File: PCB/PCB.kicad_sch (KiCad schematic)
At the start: 45 parts, among them J1 6V, J10 GND, J11 GND, J12 VBUS, J13 GND, J14 3V3, J15 6V, J16 GND, J2 GND, J3 12V, J4 GND, J5 vREF, J6 GND, J7 6V, J8 5V, J9 GND, U1 TPS565208, U2 OPA192ID, U3 ADP7142AUJZ-5.0, U4 MCP1826S-3302E/DB

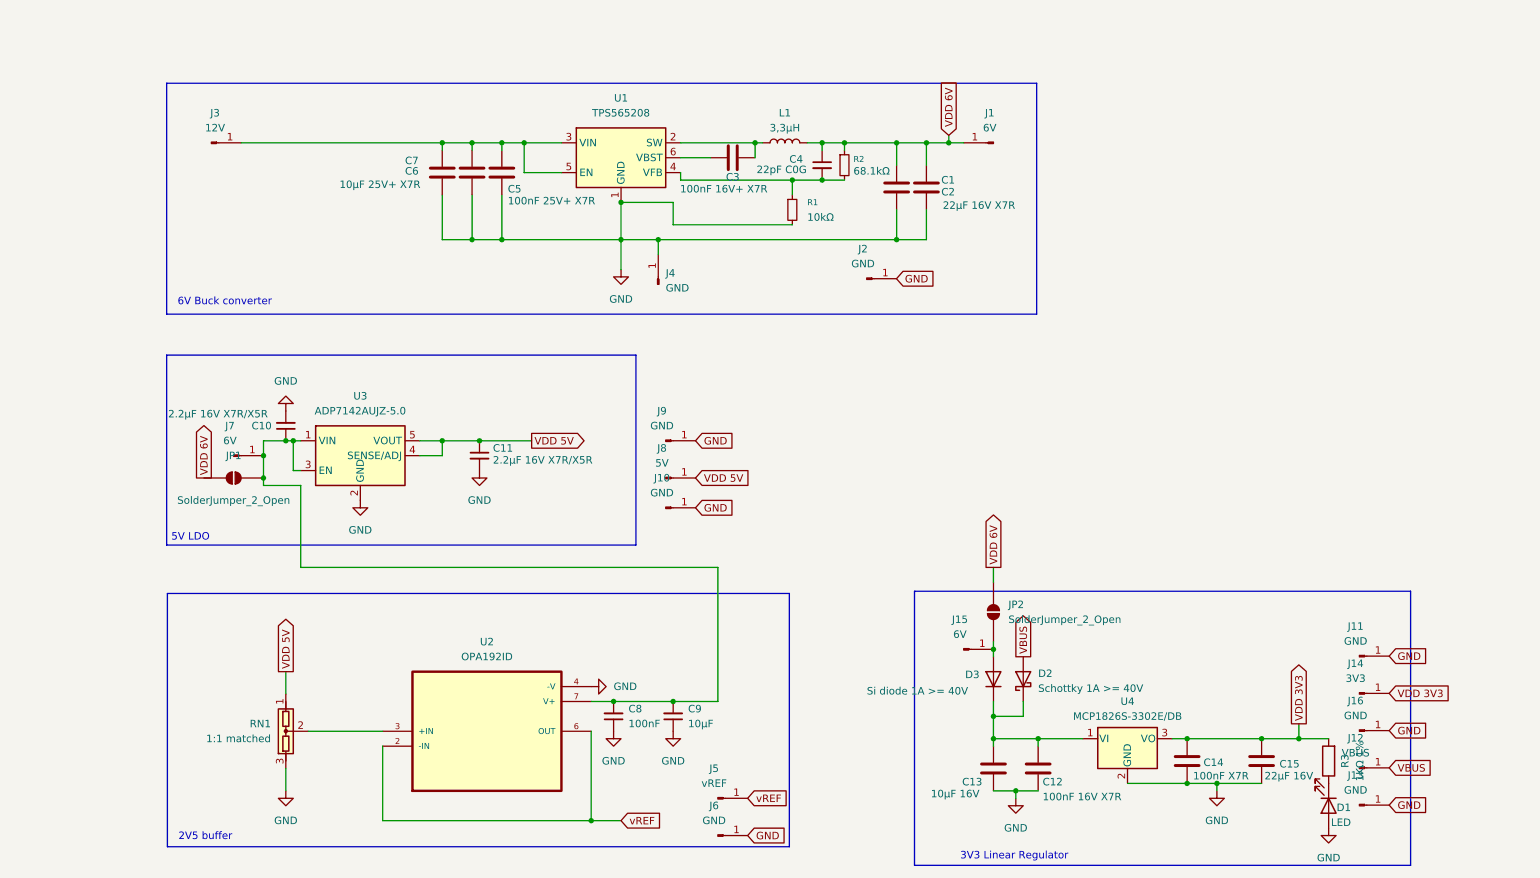
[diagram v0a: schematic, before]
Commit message: schematic rethought
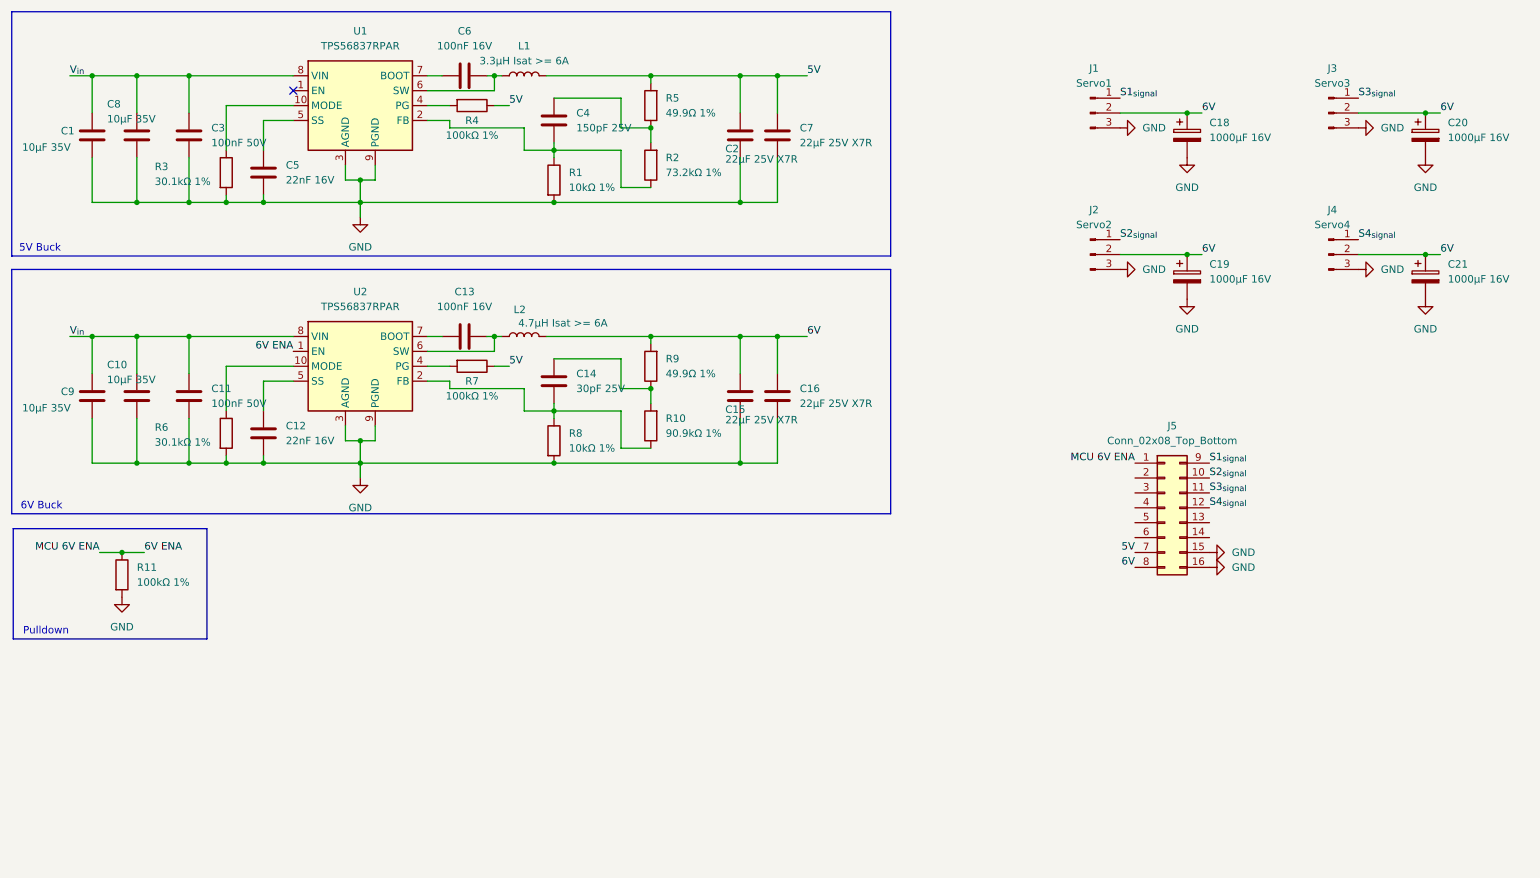
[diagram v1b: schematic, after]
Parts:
- removed C10, C11: 2.2µF 16V X7R/X5R, Capacitor_SMD:C_0805_2012Metric, symbol Device:C_Small
- removed C4: 22pF C0G, Capacitor_SMD:C_0603_1608Metric, symbol Device:C_Small
- removed C8: 100nF, Capacitor_SMD:C_0603_1608Metric, symbol Device:C_Small
- removed C9: 10µF, Capacitor_SMD:C_0603_1608Metric, symbol Device:C_Small
- removed D1: LED, LED_SMD:LED_0603_1608Metric, symbol Device:LED
- removed D2: Schottky 1A >= 40V, Diode_SMD:D_SMA, symbol Device:D_Schottky
- removed D3: Si diode 1A >= 40V, Diode_SMD:D_SMA, symbol Device:D
- removed J1, J15, J7: 6V, Connector_Wire:SolderWirePad_1x01_SMD_1x2mm, symbol Connector:Conn_01x01_Pin
- removed J10, J11, J13, J16, J2, J4, J6, J9: GND, Connector_Wire:SolderWirePad_1x01_SMD_1x2mm, symbol Connector:Conn_01x01_Pin
- removed J12: VBUS, Connector_Wire:SolderWirePad_1x01_SMD_1x2mm, symbol Connector:Conn_01x01_Pin
- removed J14: 3V3, Connector_Wire:SolderWirePad_1x01_SMD_1x2mm, symbol Connector:Conn_01x01_Pin
- removed J3: 12V, Connector_Wire:SolderWirePad_1x01_SMD_1x2mm, symbol Connector:Conn_01x01_Pin
- removed J5: vREF, Connector_Wire:SolderWirePad_1x01_SMD_1x2mm, symbol Connector:Conn_01x01_Pin
- removed J8: 5V, Connector_Wire:SolderWirePad_1x01_SMD_1x2mm, symbol Connector:Conn_01x01_Pin
- removed JP1, JP2: SolderJumper_2_Open, Jumper:SolderJumper-2_P1.3mm_Open_RoundedPad1.0x1.5mm, symbol Jumper:SolderJumper_2_Open
- removed R1: 10kΩ, Resistor_SMD:R_0603_1608Metric, symbol Device:R_Small
- removed R2: 68.1kΩ, Resistor_SMD:R_0603_1608Metric, symbol Device:R_Small
- removed RN1: 1:1 matched, Package_TO_SOT_SMD:SOT-23, symbol Device:VoltageDivider
- removed U1: TPS565208, Package_TO_SOT_SMD:TSOT-23-6, symbol Regulator_Switching:TPS565208
- removed U2: OPA192ID, Package_SO:SOIC-8_3.9x4.9mm_P1.27mm, symbol custom_sym:OPA192ID
- removed U3: ADP7142AUJZ-5.0, Package_TO_SOT_SMD:TSOT-23-5, symbol Regulator_Linear:ADP7142AUJZ-5.0
- removed U4: MCP1826S-3302E/DB, Package_TO_SOT_SMD:SOT-223-3_TabPin2, symbol Regulator_Linear:MCP1826S
- added C10, C8, C9: 10µF 35V, symbol Device:C
- added C11: 100nF 50V, symbol Device:C
- added C16: 22µF 25V X7R, symbol Device:C
- added C18, C19, C20, C21: 1000µF 16V, symbol Device:C_Polarized
- added C4: 150pF 25V, symbol Device:C
- added J1: Servo1, symbol Connector:Conn_01x03_Pin
- added J2: Servo2, symbol Connector:Conn_01x03_Pin
- added J3: Servo3, symbol Connector:Conn_01x03_Pin
- added J4: Servo4, symbol Connector:Conn_01x03_Pin
- added J5: Conn_02x08_Top_Bottom, symbol Connector_Generic:Conn_02x08_Top_Bottom
- added L2: 4.7µH Isat >= 6A, symbol Device:L
- added R1, R8: 10kΩ 1%, symbol Device:R
- added R10: 90.9kΩ 1%, symbol Device:R
- added R11, R4, R7: 100kΩ 1%, symbol Device:R
- added R2: 73.2kΩ 1%, symbol Device:R
- added R5, R9: 49.9Ω 1%, symbol Device:R
- added R6: 30.1kΩ 1%, symbol Device:R
- added U1, U2: TPS56837RPAR, das-boot:TPS5683x_VQFN-HR-10_3x3mm_RPA0010A, symbol das-boot:TPS56837RPAR
- C1: value 22µF 16V X7R -> 10µF 35V; footprint Capacitor_SMD:C_0805_2012Metric -> (none); KiLib_Generator SMD_2terminal_chip_molded -> (none)
- C12: value 100nF 16V X7R -> 22nF 16V; footprint Capacitor_SMD:C_0805_2012Metric -> (none); KiLib_Generator SMD_2terminal_chip_molded -> (none)
- C13: value 10µF 16V -> 100nF 16V; footprint Capacitor_SMD:C_0805_2012Metric -> (none); KiLib_Generator SMD_2terminal_chip_molded -> (none)
- C14: value 100nF X7R -> 30pF 25V; footprint Capacitor_SMD:C_0805_2012Metric -> (none); KiLib_Generator SMD_2terminal_chip_molded -> (none)
- C15: value 22µF 16V -> 22µF 25V X7R; footprint Capacitor_SMD:C_0805_2012Metric -> (none); KiLib_Generator SMD_2terminal_chip_molded -> (none)
- C2: value 22µF 16V X7R -> 22µF 25V X7R; footprint Capacitor_SMD:C_0805_2012Metric -> (none); KiLib_Generator SMD_2terminal_chip_molded -> (none)
- C3: value 100nF 16V+ X7R -> 100nF 50V; footprint Capacitor_SMD:C_0603_1608Metric -> (none); KiLib_Generator SMD_2terminal_chip_molded -> (none)
- C5: value 100nF 25V+ X7R -> 22nF 16V; footprint Capacitor_SMD:C_0603_1608Metric -> (none); KiLib_Generator SMD_2terminal_chip_molded -> (none)
- C6: value 10µF 25V+ X7R -> 100nF 16V; footprint Capacitor_SMD:C_0805_2012Metric -> (none); KiLib_Generator SMD_2terminal_chip_molded -> (none)
- C7: value 10µF 25V+ X7R -> 22µF 25V X7R; footprint Capacitor_SMD:C_0805_2012Metric -> (none); KiLib_Generator SMD_2terminal_chip_molded -> (none)
- L1: value 3,3µH -> 3.3µH Isat >= 6A; footprint Inductor_SMD:L_Coilcraft_XAL5030-XXX -> (none); KiLib_Generator inductor/SMD -> (none)
- R3: value 1KΩ 1% -> 30.1kΩ 1%; footprint Resistor_SMD:R_0603_1608Metric -> (none); KiLib_Generator SMD_2terminal_chip_molded -> (none)
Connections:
- net GND: now also C1.2, C2.2, C3.2, R3.2, C10.2, C11.2, C16.2, C18.2, C19.2, C20.2, C21.2, C8.2, C9.2, J1.3 (Pin_3), J2.3 (Pin_3), J3.3 (Pin_3), J4.3 (Pin_3), J5.15 (Pin_15), J5.16 (Pin_16), R1.2, R11.2, R6.2, R8.2, U1.3 (AGND), U1.9 (PGND), U2.3 (AGND), U2.9 (PGND); no longer C1.1, C13.2, C14.1, C2.1, C6.2
- net V_{in}: now reaches C3.1
- net V_{in}: now also C1.1, C10.1, C11.1, C8.1, C9.1, U1.8 (VIN), U2.8 (VIN)
- net at L1.1: now also C6.2, U1.6 (SW); no longer C3.2
- net at C13.1: now also U2.7 (BOOT); no longer C12.1
- net at R3.1: now also U1.10 (MODE)
- removed net VDD 3V3: C14.2, C15.1, R3.2
- removed net VDD 6V: C1.2, C2.2, L1.2
- new net: C14.1, R10.2, R9.1
- new net: C5.1, U1.5 (SS)
- new net: R7.2, U2.4 (PG)
- new net: C4.1, R2.2, R5.1
- new net: C4.2, R1.1, R2.1, U1.2 (FB)
- new net: R4.2, U1.4 (PG)
- new net: C13.2, L2.1, U2.6 (SW)
- new net: R6.1, U2.10 (MODE)
- new net: C14.2, R10.1, R8.1, U2.2 (FB)
- new net: C12.1, U2.5 (SS)
- new net: C6.1, U1.7 (BOOT)
- new net 5V: C2.1, C7.1, J5.7 (Pin_7), L1.2, R4.1, R5.2, R7.1
- new net 6V: C15.1, C16.1, C18.1, C19.1, C20.1, C21.1, J1.2 (Pin_2), J2.2 (Pin_2), J3.2 (Pin_2), J4.2 (Pin_2), J5.8 (Pin_8), L2.2, R9.2
- new net 6V ENA: J5.1 (Pin_1), R11.1, U2.1 (EN)
- new net S1_{signal}: J1.1 (Pin_1), J5.9 (Pin_9)
- new net S2_{signal}: J2.1 (Pin_1), J5.10 (Pin_10)
- new net S3_{signal}: J3.1 (Pin_1), J5.11 (Pin_11)
- new net S4_{signal}: J4.1 (Pin_1), J5.12 (Pin_12)
- no-connect marks 0 -> 1
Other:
- note added: "5V Buck"
- note added: "6V Buck"
- note added: "Pulldown"
- note removed: "2V5 buffer"
- note removed: "3V3 Linear Regulator"
- note removed: "5V LDO"
- note removed: "6V Buck converter"
